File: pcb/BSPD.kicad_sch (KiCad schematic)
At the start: 50 parts, among them J1 Test header, J2 T4142012121-000, Q1 AO3400A, U1 LM339, U2 LM339, U3 74HC32, U4 74HC02

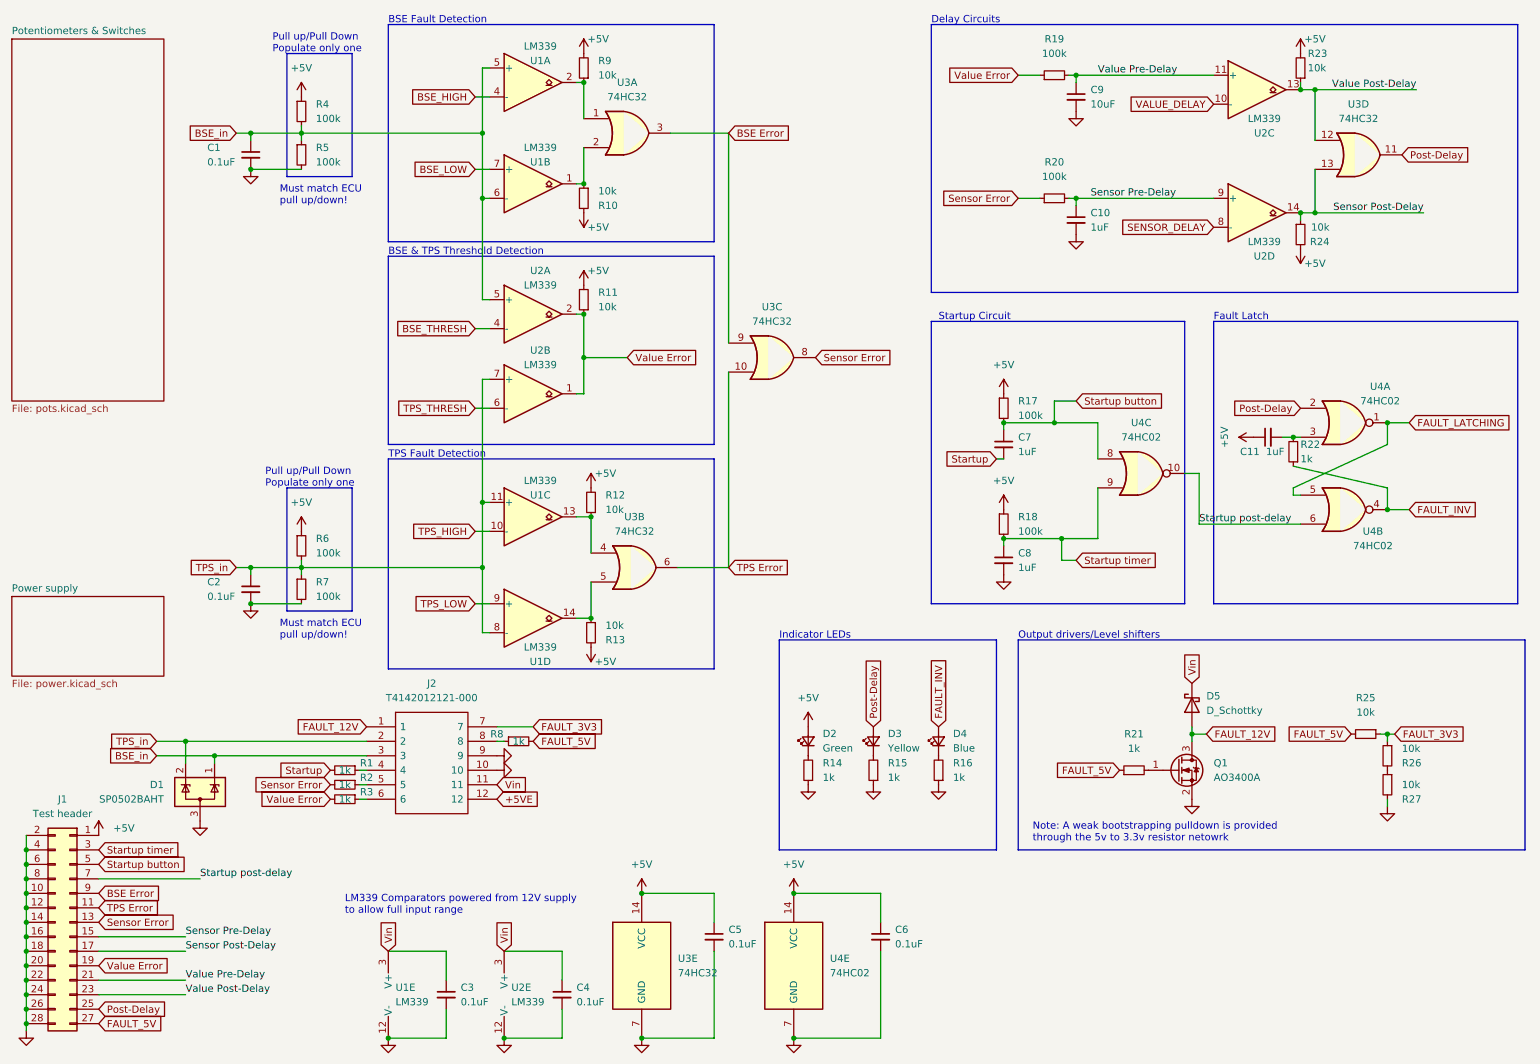
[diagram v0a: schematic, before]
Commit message: CI/CD Changes
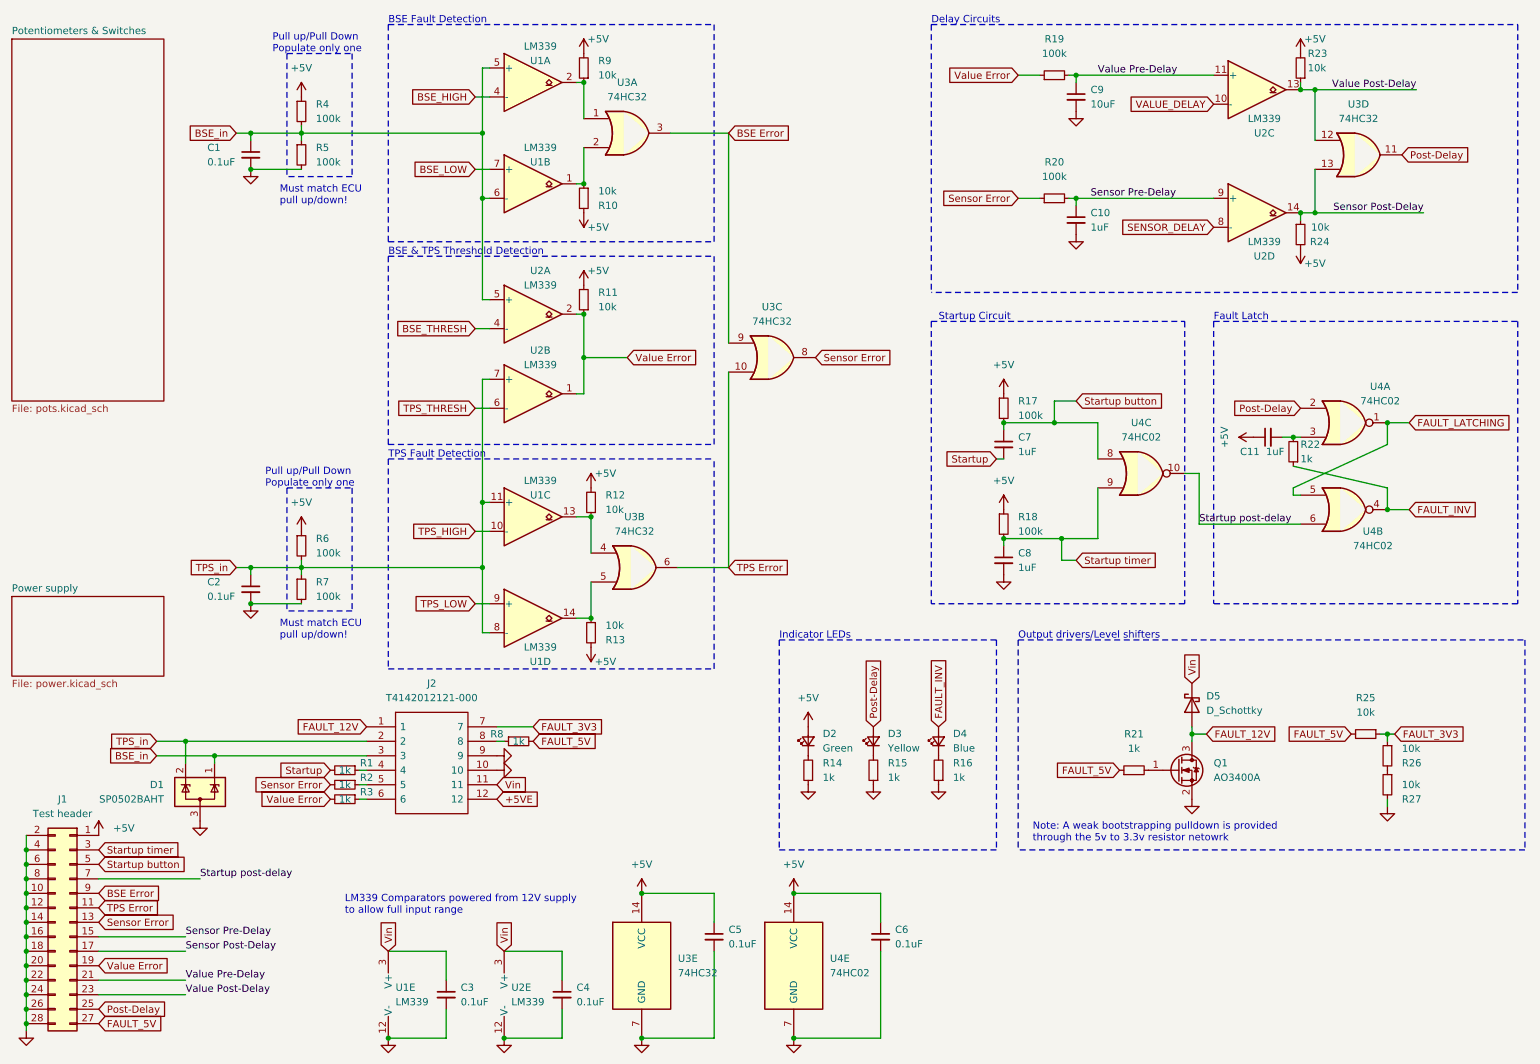
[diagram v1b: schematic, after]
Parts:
- C1, C2, C3, C4, C5, C6: Spice_Model 0.1u -> (none); Spice_Netlist_Enabled Y -> (none); Spice_Primitive C -> (none)
- C10, C11, C7, C8: Spice_Model 1u -> (none); Spice_Netlist_Enabled Y -> (none); Spice_Primitive C -> (none)
- C9: Spice_Model 10u -> (none); Spice_Netlist_Enabled Y -> (none); Spice_Primitive C -> (none)
- D1: Spice_Model SP0502BAHT -> (none); Spice_Netlist_Enabled N -> (none); Spice_Primitive D -> (none)
- D5: Spice_Model D_Schottky -> (none); Spice_Netlist_Enabled N -> (none); Spice_Primitive D -> (none)
- R10, R11, R12, R13, R23, R24, R25, R26, R27, R9: Spice_Model 10k -> (none); Spice_Netlist_Enabled Y -> (none); Spice_Primitive R -> (none)
- R17, R18, R19, R20, R4, R6: Spice_Model 100k -> (none); Spice_Netlist_Enabled Y -> (none); Spice_Primitive R -> (none)
- R5, R7: Spice_Model 100k -> (none); Spice_Netlist_Enabled N -> (none); Spice_Primitive R -> (none)
- U1, U2: Spice_Lib_File SPICE models/lmx39_spice.lib -> (none); Spice_Model LM339 -> (none); Spice_Netlist_Enabled Y -> (none); Spice_Primitive X -> (none)
- U3: Spice_Lib_File SPICE models/74hc32.lib -> (none); Spice_Model 74HC32_pkg -> (none); Spice_Netlist_Enabled Y -> (none); Spice_Primitive X -> (none)
- U4: Spice_Lib_File SPICE models/74hc02.lib -> (none); Spice_Model 74HC02_pkg -> (none); Spice_Netlist_Enabled Y -> (none); Spice_Primitive X -> (none)
